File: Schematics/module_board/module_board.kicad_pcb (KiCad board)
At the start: 2 copper layers, 35 x 35 mm, 30 parts, among them J1 Conn_01x01_Male, J10 Conn_01x01_Male, J2 Conn_01x01_Male, J3 Conn_01x01_Male, J4 Conn_01x01_Male, J5 Conn_01x01_Male, J6 Conn_01x01_Male, J7 Conn_01x01_Male, J8 Conn_01x01_Male, J9 Conn_01x01_Male, U1 RP2040, U2 W25Q16JVSSIQ, Y1 ABLS-12.000MHZ-B4-T

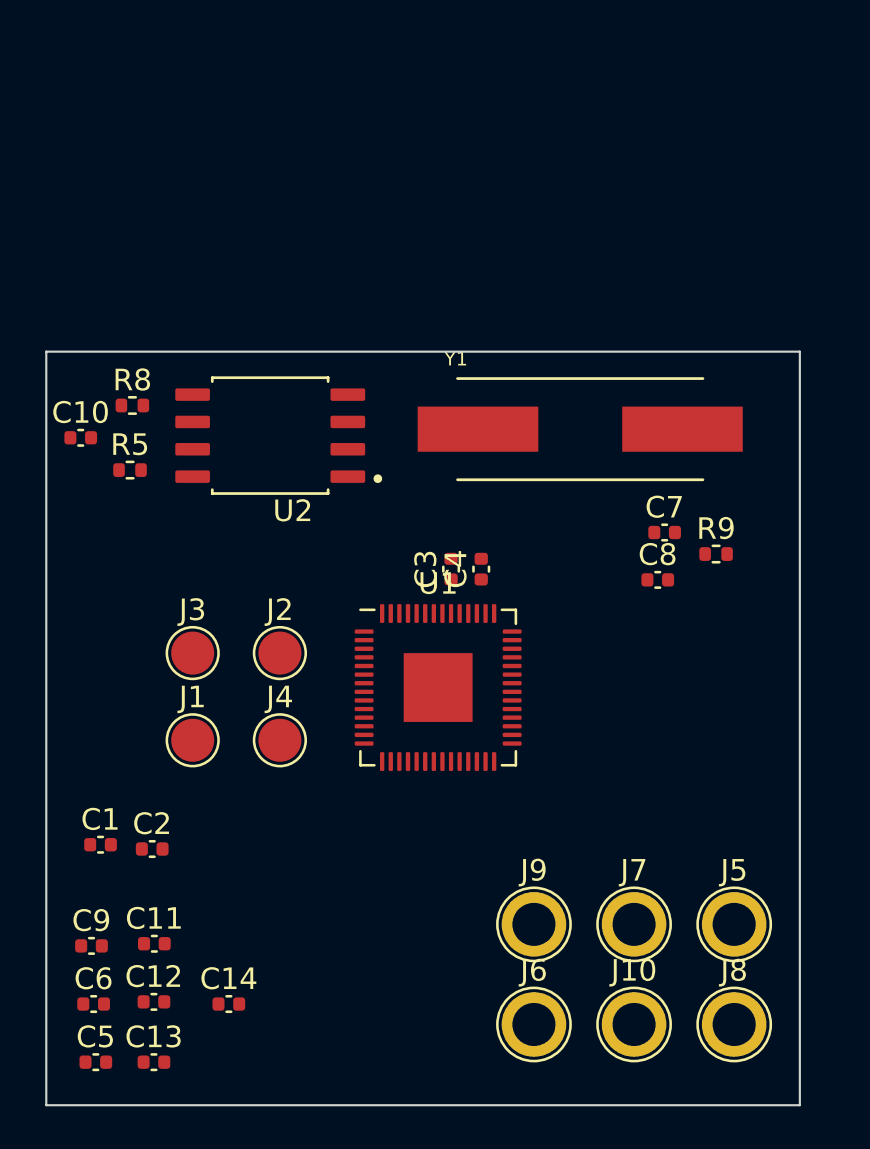
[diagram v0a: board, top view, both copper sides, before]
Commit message: Completed non-routed Rough PCB Draft
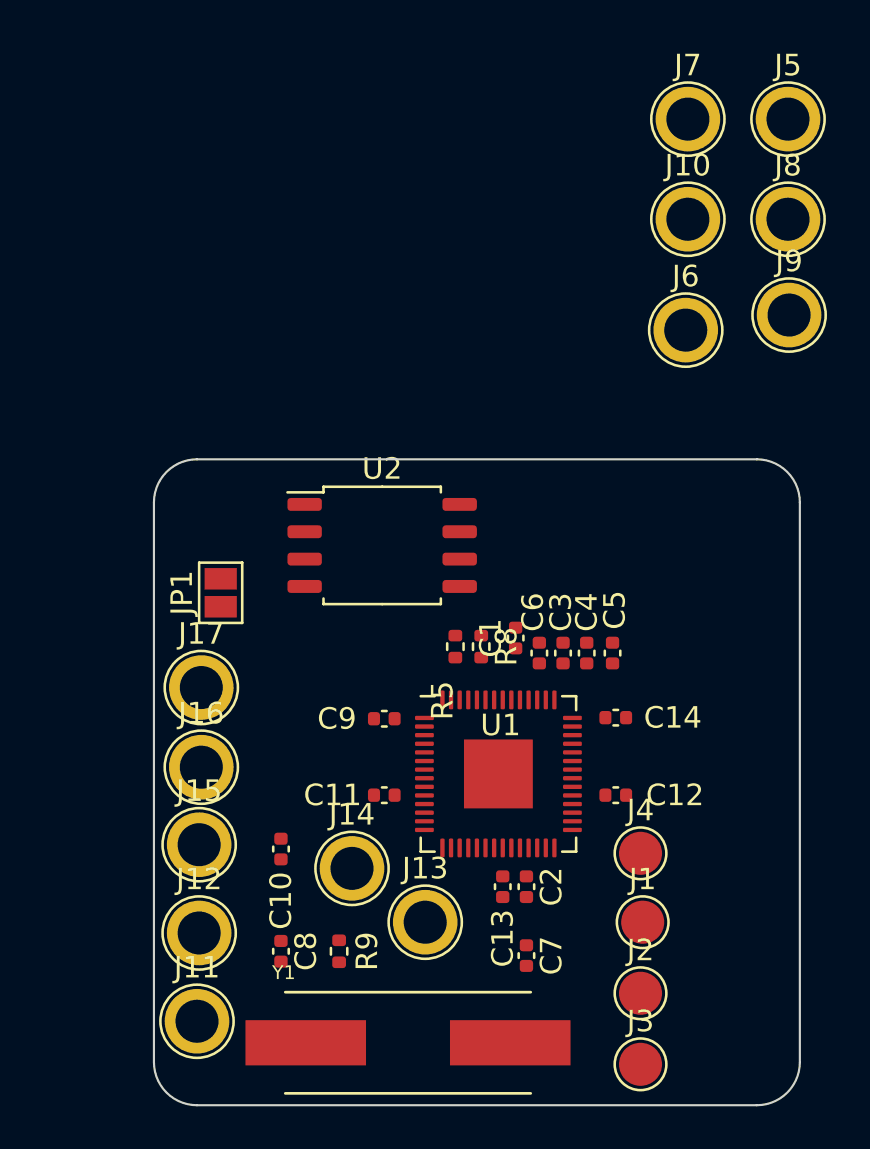
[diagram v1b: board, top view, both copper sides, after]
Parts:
- added J11: Conn_01x01_Male, TestPoint:TestPoint_Plated_Hole_D2.0mm, F.Cu at (147.0, 101.1)
- added J12: Conn_01x01_Male, TestPoint:TestPoint_Plated_Hole_D2.0mm, F.Cu at (147.1, 97.0)
- added J13: Conn_01x01_Male, TestPoint:TestPoint_Plated_Hole_D2.0mm, F.Cu at (157.6, 96.5)
- added J14: Conn_01x01_Male, TestPoint:TestPoint_Plated_Hole_D2.0mm, F.Cu at (154.2, 94.0)
- added J15: Conn_01x01_Male, TestPoint:TestPoint_Plated_Hole_D2.0mm, F.Cu at (147.1, 92.9)
- added J16: Conn_01x01_Male, TestPoint:TestPoint_Plated_Hole_D2.0mm, F.Cu at (147.2, 89.3)
- added J17: Conn_01x01_Male, TestPoint:TestPoint_Plated_Hole_D2.0mm, F.Cu at (147.2, 85.6)
- added JP1: Jumper_2_Open, Jumper:SolderJumper-2_P1.3mm_Open_Pad1.0x1.5mm, F.Cu at (148.1, 81.2)
- U2: footprint W25Q16JVSSIQ:SOIC127P790X216-8N -> Package_SO:SOIC-8_5.23x5.23mm_P1.27mm
- moved J10 37.5 mm to (169.8, 63.9)
- moved J8 37.5 mm to (174.4, 63.9)
- moved J5 37.5 mm to (174.4, 59.2)
- moved J7 37.5 mm to (169.8, 59.2)
- moved J6 33.0 mm to (169.7, 69.0)
- moved J9 30.7 mm to (174.5, 68.3)
- moved C5 30.6 mm to (166.3, 84.0), turned to 90 degrees
- moved Y1 29.6 mm to (156.8, 102.1)
- moved J3 28.2 mm to (167.6, 103.1)
- moved C6 26.3 mm to (162.9, 84.0), turned to 90 degrees
- moved R9 25.4 mm to (153.6, 97.8), turned to 90 degrees
- moved C8 24.6 mm to (150.9, 97.8), turned to -90 degrees
- moved C12 23.5 mm to (166.4, 90.6)
- moved J2 23.0 mm to (167.6, 99.8)
- moved J1 22.5 mm to (167.7, 96.5)
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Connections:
- C3 pad 1: +1V1 -> GND
- C3 pad 2: GND -> +1V1
- U1 pad 11: /GPIO8 -> /SPI1_RX
- U1 pad 12: /GPIO9 -> /SPI1_CS_IO9
- U1 pad 13: /GPIO10 -> /SPI1_SCK
- U1 pad 14: /GPIO11 -> /SPI1_TX
- U1 pad 27: /GPIO16 -> /RX
- U1 pad 28: /GPIO17 -> /CS
- U1 pad 29: /GPIO18 -> /SCLK
- U1 pad 30: /GPIO19 -> /TX
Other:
- board size 35 x 35 mm -> 30 x 30 mm
